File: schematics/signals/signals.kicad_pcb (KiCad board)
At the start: 4 copper layers, 38.1 x 34.9 mm, 42 parts, among them J1 Sensors, J2 Conditioned, SW1 Returns, SW2 Feedbacks, SW3 Returns, SW4 Feedbacks, U1 AD8422ARMZ, U2 OPA2182, U3 AD8422ARMZ

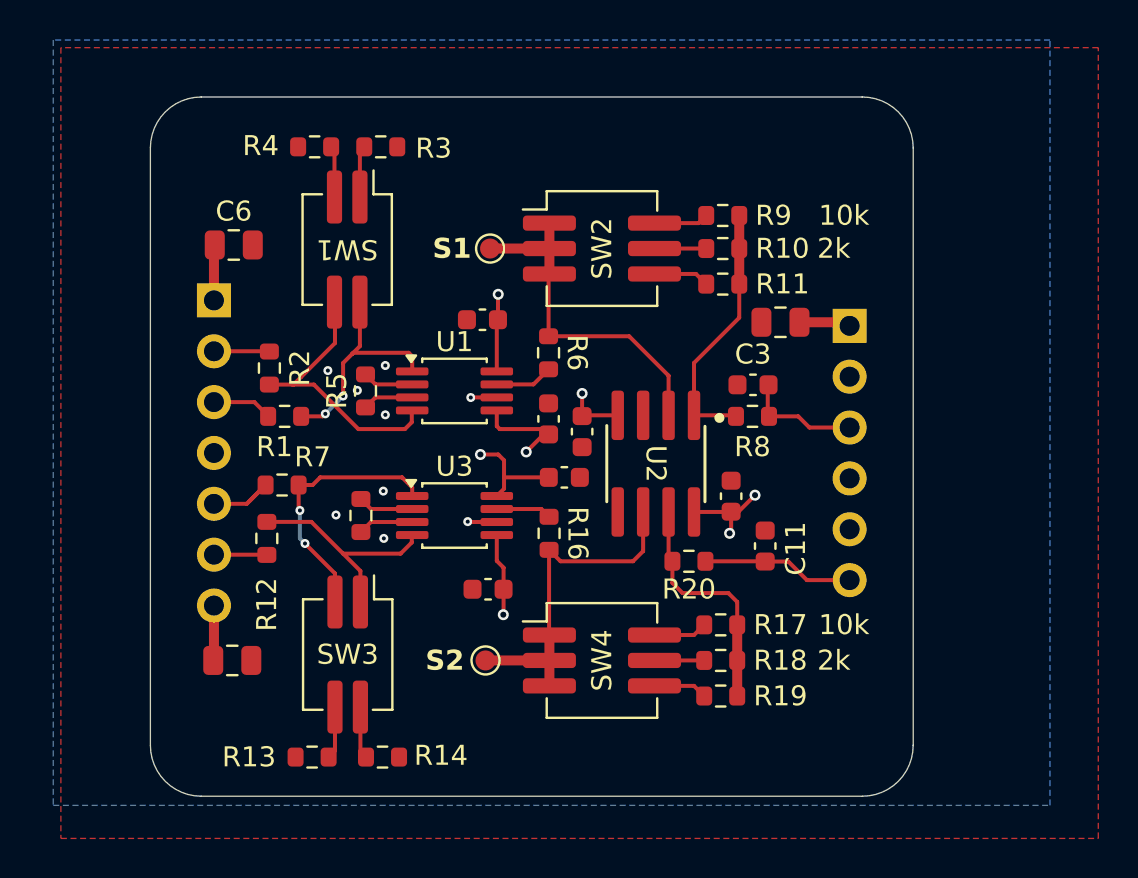
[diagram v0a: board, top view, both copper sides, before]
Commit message: feat(signals): bessel filter
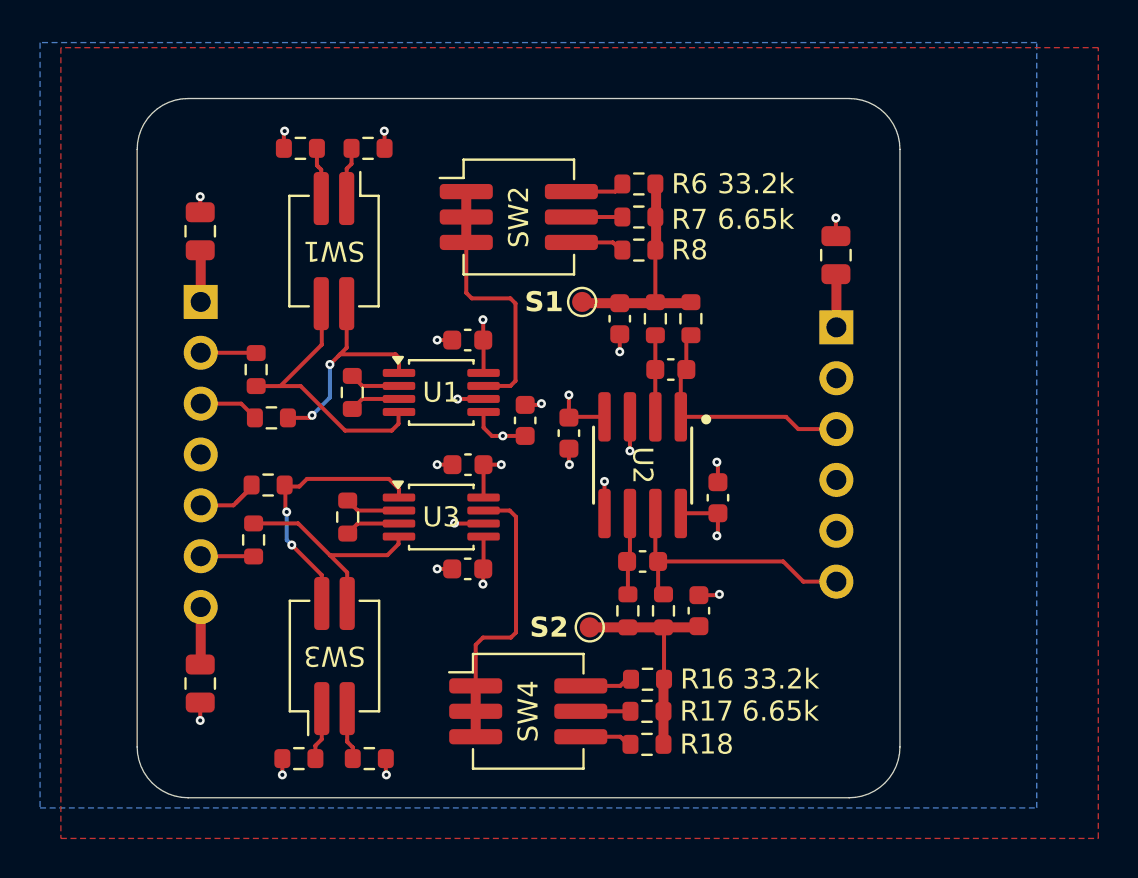
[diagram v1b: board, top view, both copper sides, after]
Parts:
- added C12: 220pF, Capacitor_SMD:C_0603_1608Metric, F.Cu at (204.6, 68.8)
- added C13: 100pF, Capacitor_SMD:C_0603_1608Metric, F.Cu at (201.8, 66.3)
- C11: value 0.62nF -> 0.1uF
- C3: value 0.62nF -> 100pF
- C9: value 0.1uF -> 220pF
- R10: value 2k -> 6.65k
- R11: value Rf -> 100
- R16, R6: value 10k -> 33.2k
- R17, R9: value 10k -> 6.65k
- R18: value 2k -> ~
- R19: value Rf -> 6.65k
- R20: value 1k -> 6.65k
- R7: value 100 -> 6.65k
- R8: value 1k -> ~
- moved R11 24.8 mm to (183.1, 62.5)
- moved R7 22.3 mm to (201.6, 49.1)
- moved C11 15.4 mm to (193.1, 61.5), turned to 180 degrees
- moved C9 15.0 mm to (200.6, 54.2), turned to 90 degrees
- moved R8 10.1 mm to (201.6, 50.7)
- moved R6 9.56 mm to (201.6, 47.4), turned to 0 degrees
- moved R16 8.79 mm to (202.0, 72.2), turned to 0 degrees
- moved C10 6.65 mm to (193.0, 66.7), turned to 180 degrees
- moved R19 6.29 mm to (201.0, 68.8), turned to 90 degrees
- moved R17 5.67 mm to (202.0, 73.8)
- moved R18 5.58 mm to (202.0, 75.4)
- moved TP2 5.46 mm to (199.1, 69.6)
- moved R9 5.40 mm to (204.2, 54.2), turned to -90 degrees
- moved TP1 5.31 mm to (198.8, 53.3)
- moved R10 4.86 mm to (202.4, 54.2), turned to -90 degrees
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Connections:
- C10 pad 1: +12V -> -3V3
- C11 pad 1: /Sc2- -> +12V
- C3 pad 1: /Sc1- -> Net-(U2A--)
- C3 pad 2: GND -> /Sc1-
- C9 pad 1: -3V3 -> GND
- C9 pad 2: GND -> Net-(C9-Pad2)
- R10 pad 1: Net-(R10-Pad1) -> Net-(C9-Pad2)
- R10 pad 2: Net-(R10-Pad2) -> Net-(U2A--)
- R11 pad 1: Net-(R11-Pad1) -> /S2-
- R11 pad 2: Net-(R10-Pad2) -> Net-(U3--)
- R16 pad 2: Net-(U2B--) -> Net-(C12-Pad2)
- R17 pad 2: Net-(R17-Pad2) -> Net-(C12-Pad2)
- R18 pad 2: Net-(R17-Pad2) -> Net-(C12-Pad2)
- R19 pad 1: Net-(R19-Pad1) -> Net-(C12-Pad2)
- R19 pad 2: Net-(R17-Pad2) -> Net-(U2B--)
- R20 pad 1: Net-(R17-Pad2) -> Net-(C12-Pad2)
- R6 pad 2: Net-(U2A--) -> Net-(C9-Pad2)
- R7 pad 1: /S2- -> Net-(R7-Pad1)
- R7 pad 2: Net-(U3--) -> Net-(C9-Pad2)
- R8 pad 1: Net-(R10-Pad2) -> Net-(R8-Pad1)
- R8 pad 2: /Sc1- -> Net-(C9-Pad2)
- R9 pad 1: Net-(R9-Pad1) -> Net-(C9-Pad2)
- R9 pad 2: Net-(R10-Pad2) -> /Sc1-
- SW2 pad 1: Net-(U2A--) -> Net-(SW2-Pad1)
- SW2 pad 2: Net-(U2A--) -> Net-(SW2-Pad1)
- SW2 pad 3: Net-(U2A--) -> Net-(SW2-Pad1)
- SW2 pad 4: Net-(R11-Pad1) -> Net-(R8-Pad1)
- SW2 pad 5: Net-(R10-Pad1) -> Net-(R7-Pad1)
- SW2 pad 6: Net-(R9-Pad1) -> Net-(R6-Pad1)
- SW3 pad 1: Net-(U3-+) -> Net-(R13-Pad1)
- SW3 pad 2: Net-(U3--) -> Net-(R14-Pad1)
- SW3 pad 3: Net-(R13-Pad1) -> Net-(U3-+)
- SW3 pad 4: Net-(R14-Pad1) -> Net-(U3--)
- SW4 pad 1: Net-(U2B--) -> Net-(SW4-Pad1)
- SW4 pad 2: Net-(U2B--) -> Net-(SW4-Pad1)
- SW4 pad 3: Net-(U2B--) -> Net-(SW4-Pad1)
- SW4 pad 4: Net-(R19-Pad1) -> Net-(R18-Pad1)
- SW4 pad 5: Net-(R18-Pad1) -> Net-(R17-Pad1)
- SW4 pad 6: Net-(R17-Pad1) -> Net-(R16-Pad1)
- TP1 pad 1: Net-(U2A--) -> Net-(C9-Pad2)
- TP2 pad 1: Net-(U2B--) -> Net-(C12-Pad2)
- U1 pad 7: Net-(R6-Pad1) -> Net-(SW2-Pad1)
- U2 pad 1: Net-(R10-Pad2) -> /Sc1-
- U2 pad 7: Net-(R17-Pad2) -> /Sc2-
- U3 pad 7: Net-(R16-Pad1) -> Net-(SW4-Pad1)
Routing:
- net GND: track 3.25 -> 18.9 mm, vias 9 -> 19
- net Net-(SW4-Pad1): track 0.00 -> 14.3 mm
- net Net-(U2A--): track 17.4 -> 4.08 mm
- net Net-(SW2-Pad1): track 0.00 -> 13.3 mm
- net Net-(R10-Pad2): track 13.0 -> 0.00 mm
- net Net-(U2B--): track 17.1 -> 4.11 mm
- net Net-(R17-Pad2): track 12.1 -> 0.00 mm
- net Net-(C9-Pad2): track 0.00 -> 11.9 mm
- net Net-(C12-Pad2): track 0.00 -> 11.6 mm
- net /Sc1-: track 5.92 -> 12.3 mm
- net /Sc2-: track 7.59 -> 13.5 mm
- net +12V: track 12.6 -> 8.04 mm
- net -3V3: track 14.8 -> 10.8 mm
- net Net-(R11-Pad1): track 2.79 -> 0.00 mm
- net Net-(R8-Pad1): track 0.00 -> 2.79 mm
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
